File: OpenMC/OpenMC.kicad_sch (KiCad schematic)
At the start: 4 parts, among them IC1 EFM8LB11F32E-C-QFN24, J3 Conn_01x01_Female, J4 Conn_01x06_Female, J5 Conn_01x01_Female

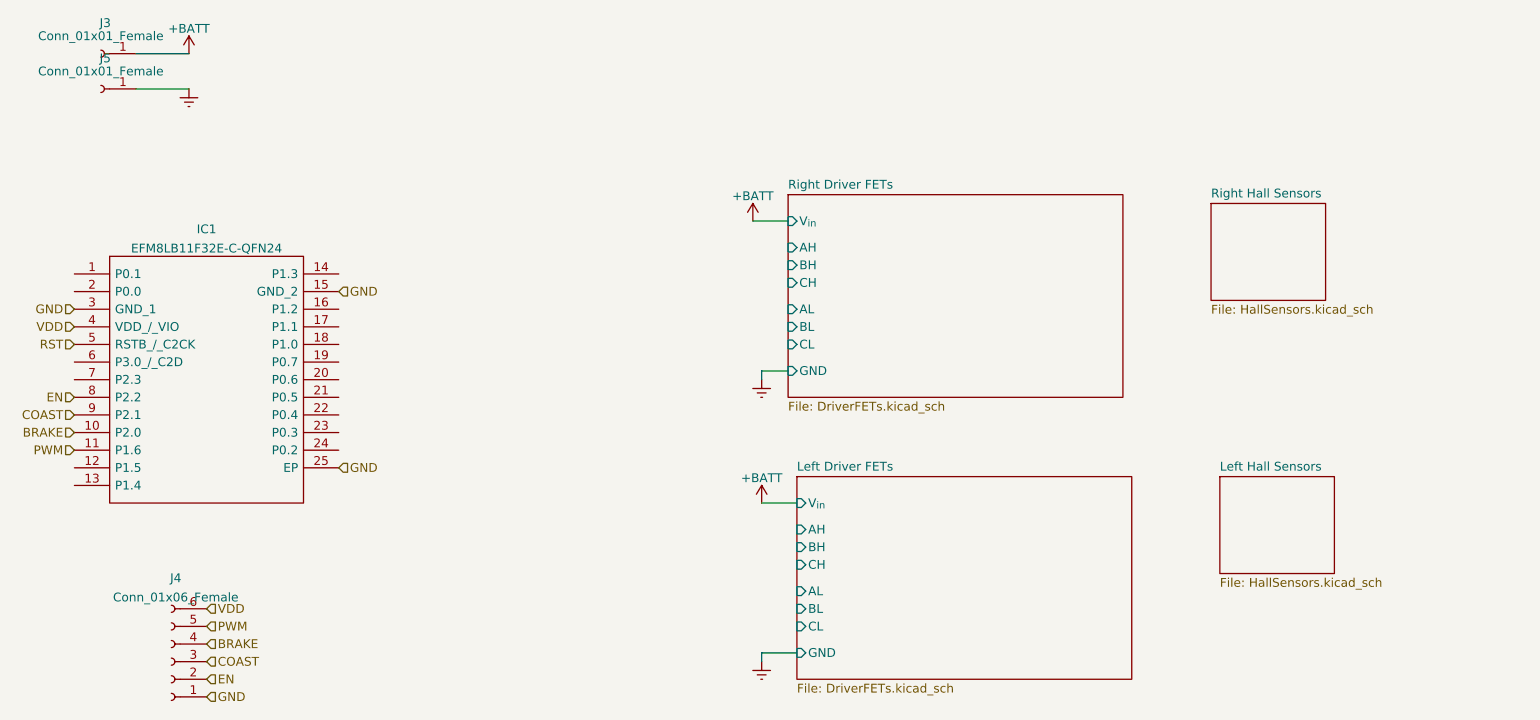
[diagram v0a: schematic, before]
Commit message: updates
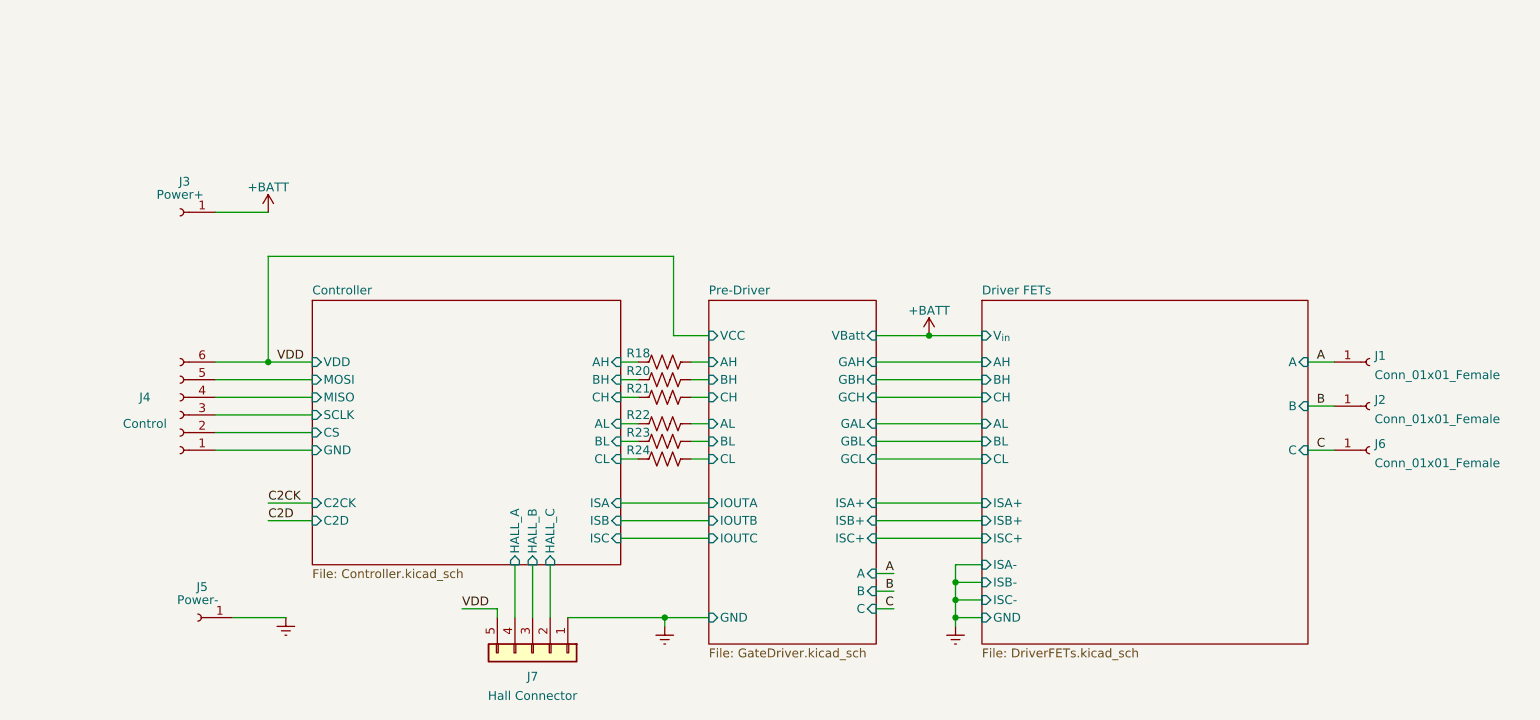
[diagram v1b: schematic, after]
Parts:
- removed IC1: EFM8LB11F32E-C-QFN24, EFM8LB11F32EBQFN24R, symbol SamacSys_Parts:EFM8LB11F32E-C-QFN24
- added J1, J2, J6: Conn_01x01_Female, Connector:Banana_Jack_1Pin, symbol Connector:Conn_01x01_Female
- added J7: Hall Connector, Connector_PinHeader_2.00mm:PinHeader_1x05_P2.00mm_Vertical, symbol Connector_Generic:Conn_01x05
- added R18, R20, R21, R22, R23, R24: R_US, Capacitor_SMD:C_0603_1608Metric, symbol Device:R_US
- J3: value Conn_01x01_Female -> Power+
- J4: value Conn_01x06_Female -> Control
- J5: value Conn_01x01_Female -> Power-
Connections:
- net Earth: now also J7.1 (Pin_1)
- net VDD: now also J7.5 (Pin_5)
- net BRAKE renamed Controller/MISO
- net COAST renamed Controller/SCLK
- net EN renamed Controller/CS
- net GND renamed Controller/GND
- net PWM renamed Controller/MOSI
- new net A: J1.1 (Pin_1)
- new net B: J2.1 (Pin_1)
- new net C: J6.1 (Pin_1)
- new net Controller/AH: R18.1
- new net Controller/AL: R22.1
- new net Controller/BH: R20.1
- new net Controller/BL: R23.1
- new net Controller/CH: R21.1
- new net Controller/CL: R24.1
- new net Controller/HALL_A: J7.4 (Pin_4)
- new net Controller/HALL_B: J7.3 (Pin_3)
- new net Controller/HALL_C: J7.2 (Pin_2)
- new net Pre-Driver/AH: R18.2
- new net Pre-Driver/AL: R22.2
- new net Pre-Driver/BH: R20.2
- new net Pre-Driver/BL: R23.2
- new net Pre-Driver/CH: R21.2
- new net Pre-Driver/CL: R24.2
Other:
- sheet Right Driver FETs renamed Driver FETs
- removed sheet Left Driver FETs
- removed sheet Left Hall Sensors
- removed sheet Right Hall Sensors
- added sheet Controller (Controller.kicad_sch)
- added sheet Pre-Driver (GateDriver.kicad_sch)
- sheet Driver FETs ports: added A, B, C, ISA+, ISA-, ISB+, ISB-, ISC+, ISC-; removed none
- moved on the sheet: J3, J4, J5
